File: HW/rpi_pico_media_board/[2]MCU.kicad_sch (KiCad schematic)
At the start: 1 part

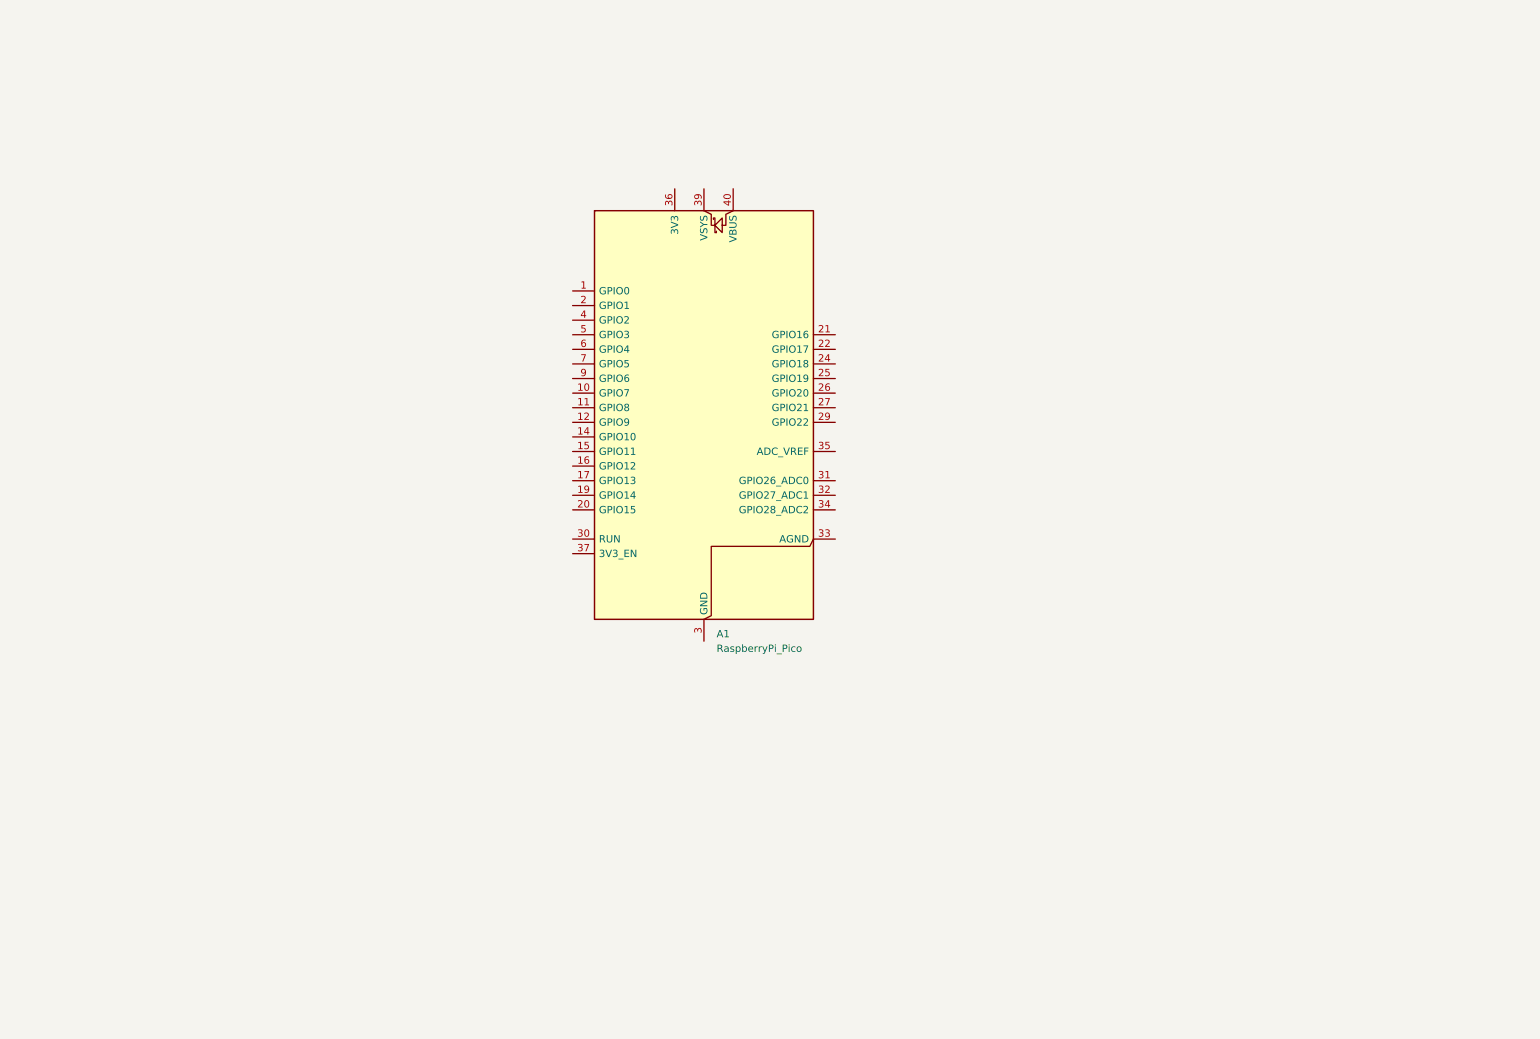
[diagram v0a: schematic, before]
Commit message: Scheme improvements
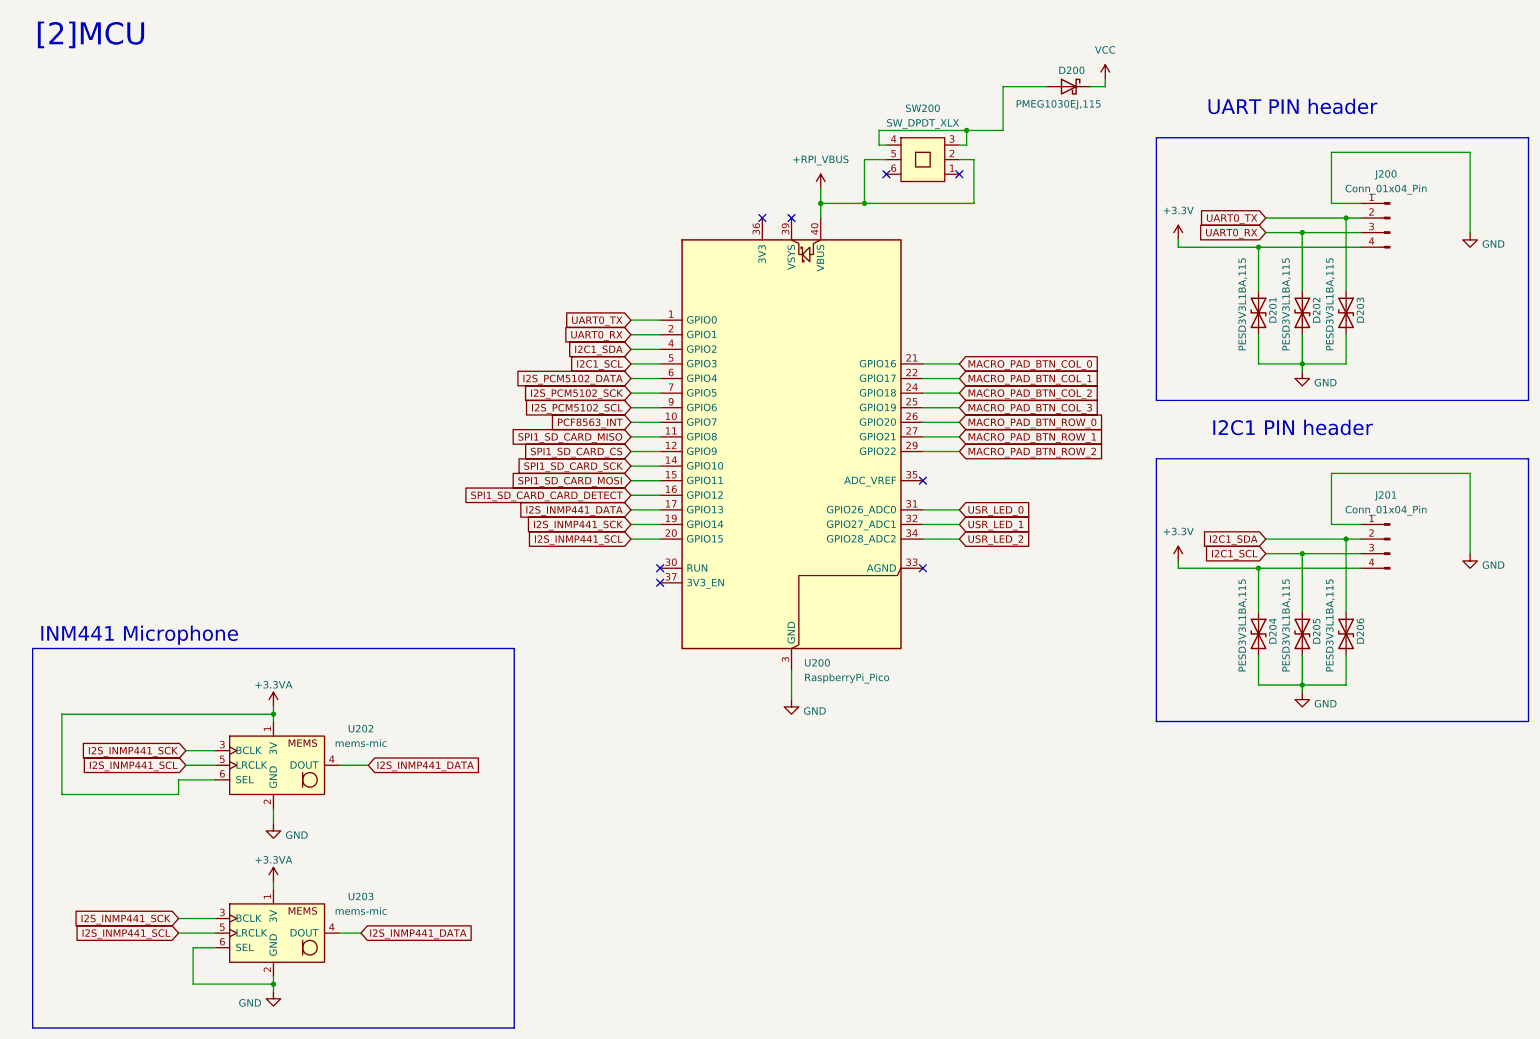
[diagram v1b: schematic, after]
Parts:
- added D200: PMEG1030EJ,115, Diode_SMD:D_SOD-323F, symbol Device:D_Schottky
- added D201, D202, D203, D204, D205, D206: PESD3V3L1BA,115, Diode_SMD:D_SOD-323, symbol Device:D_TVS
- added J200, J201: Conn_01x04_Pin, Connector_PinSocket_2.54mm:PinSocket_1x04_P2.54mm_Vertical, symbol Connector:Conn_01x04_Pin
- added SW200: SW_DPDT_XLX, rpi_pico_media_board:SW_DPDT_XLX, symbol rpi_pico_media_board:SW_DPDT_XLX
- added U202, U203: mems-mic, rpi_pico_media_board:inmp441, symbol rpi_pico_media_board:mems-mic
- renumbered A1 to U200
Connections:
- net UART0_TX: now reaches U200.1 (GPIO0)
- net UART0_TX: now also D203.1 (A1), J200.2 (Pin_2)
- net PCF8563_INT: now reaches U200.10 (GPIO7)
- net SPI1_SD_CARD_MISO: now reaches U200.11 (GPIO8)
- net SPI1_SD_CARD_CS: now reaches U200.12 (GPIO9)
- net GND: now reaches U200.13 (GND), U200.18 (GND), U200.23 (GND), U200.28 (GND), U200.3 (GND), U200.38 (GND), U200.8 (GND)
- net GND: now also D201.2 (A2), D202.2 (A2), D203.2 (A2), D204.2 (A2), D205.2 (A2), D206.2 (A2), J200.1 (Pin_1), J201.1 (Pin_1), U202.2 (GND), U203.2 (GND), U203.6 (SEL)
- net SPI1_SD_CARD_SCK: now reaches U200.14 (GPIO10)
- net SPI1_SD_CARD_MOSI: now reaches U200.15 (GPIO11)
- net SPI1_SD_CARD_CARD_DETECT: now reaches U200.16 (GPIO12)
- net I2S_INMP441_DATA: now reaches U200.17 (GPIO13)
- net I2S_INMP441_DATA: now also U202.4 (DOUT), U203.4 (DOUT)
- net I2S_INMP441_SCK: now reaches U200.19 (GPIO14)
- net I2S_INMP441_SCK: now also U202.3 (BCLK), U203.3 (BCLK)
- net UART0_RX: now reaches U200.2 (GPIO1)
- net UART0_RX: now also D202.1 (A1), J200.3 (Pin_3)
- net I2S_INMP441_SCL: now reaches U200.20 (GPIO15)
- net I2S_INMP441_SCL: now also U202.5 (LRCLK), U203.5 (LRCLK)
- net MACRO_PAD_BTN_COL_0: now reaches U200.21 (GPIO16)
- net MACRO_PAD_BTN_COL_1: now reaches U200.22 (GPIO17)
- net MACRO_PAD_BTN_COL_2: now reaches U200.24 (GPIO18)
- net MACRO_PAD_BTN_COL_3: now reaches U200.25 (GPIO19)
- net MACRO_PAD_BTN_ROW_0: now reaches U200.26 (GPIO20)
- net MACRO_PAD_BTN_ROW_1: now reaches U200.27 (GPIO21)
- net MACRO_PAD_BTN_ROW_2: now reaches U200.29 (GPIO22)
- net USR_LED_0: now reaches U200.31 (GPIO26_ADC0)
- net USR_LED_1: now reaches U200.32 (GPIO27_ADC1)
- net USR_LED_2: now reaches U200.34 (GPIO28_ADC2)
- net I2C1_SDA: now reaches U200.4 (GPIO2)
- net I2C1_SDA: now also D206.1 (A1), J201.2 (Pin_2)
- net +RPI_VBUS: now reaches U200.40 (VBUS)
- net +RPI_VBUS: now also SW200.2, SW200.5
- net I2C1_SCL: now reaches U200.5 (GPIO3)
- net I2C1_SCL: now also D205.1 (A1), J201.3 (Pin_3)
- net I2S_PCM5102_DATA: now reaches U200.6 (GPIO4)
- net I2S_PCM5102_SCK: now reaches U200.7 (GPIO5)
- net I2S_PCM5102_SCL: now reaches U200.9 (GPIO6)
- new net: D200.2 (A), SW200.3, SW200.4
- new net +3.3V: D201.1 (A1), D204.1 (A1), J200.4 (Pin_4), J201.4 (Pin_4)
- new net +3.3VA: U202.1 (3V), U202.6 (SEL), U203.1 (3V)
- new net VCC: D200.1 (K)
- no-connect marks 0 -> 8
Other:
- note added: "I2C1 PIN header"
- note added: "INM441 Microphone"
- note added: "UART PIN header"
- note added: "[2]MCU"
- moved on the sheet: U200
